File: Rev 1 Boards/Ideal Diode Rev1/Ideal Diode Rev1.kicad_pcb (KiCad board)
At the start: 2 copper layers, 78.6 x 49.5 mm, 22 parts, among them Q1 NVMFS5C404NL, U1 SN74LVC2G08, U2 LM74700

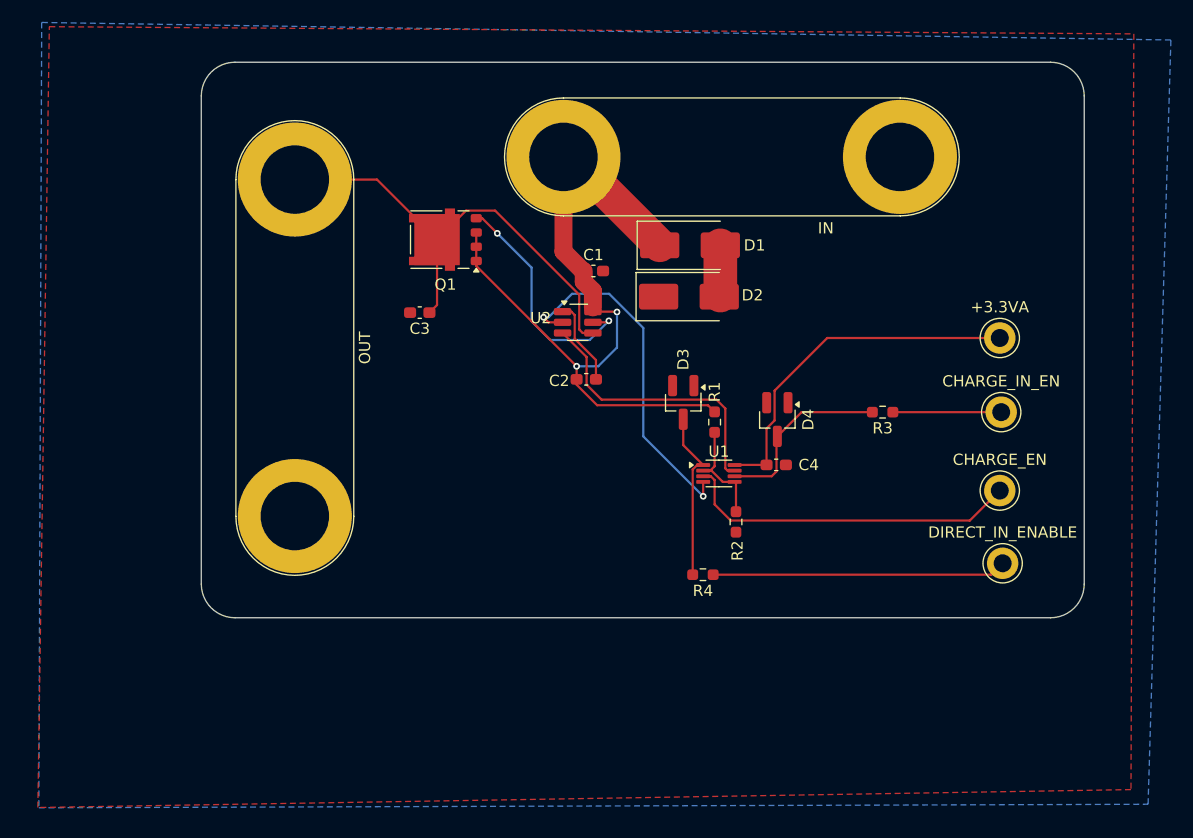
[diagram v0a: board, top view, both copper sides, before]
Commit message: ideal diode review 3 changes
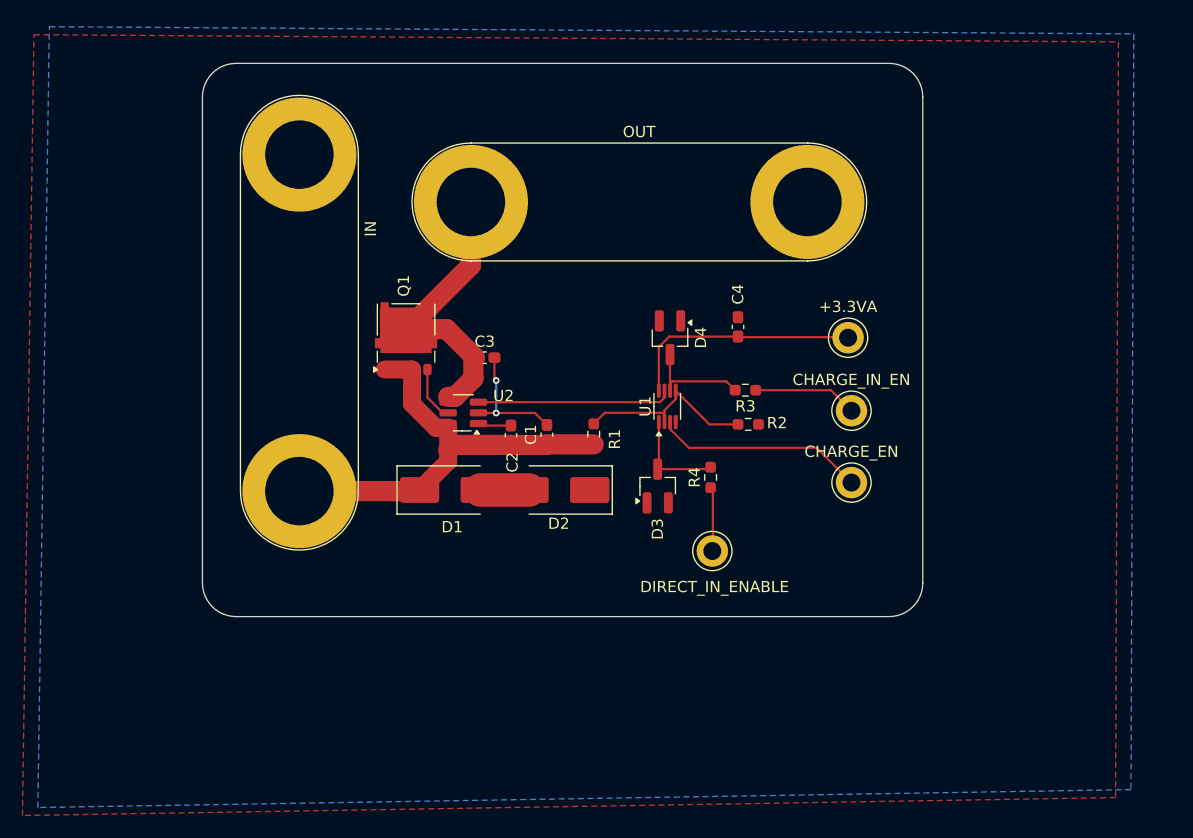
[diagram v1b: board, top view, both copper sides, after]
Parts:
- moved IN 37.9 mm to (59.8, 57.5), turned to 90 degrees
- moved D1 30.5 mm to (73.2, 57.4)
- moved DIRECT_IN_ENABLE 25.9 mm to (96.6, 62.8)
- moved G*** 23.8 mm to (90.9, 32.4)
- moved D2 20.7 mm to (82.9, 57.4), turned to 180 degrees
- moved OUT 15.8 mm to (75.1, 31.7), turned to 0 degrees
- moved C1 15.2 mm to (81.8, 52.4), turned to 90 degrees
- moved +3.3VA 13.5 mm to (108.7, 43.8)
- moved CHARGE_IN_EN 13.3 mm to (109.0, 50.3)
- moved CHARGE_EN 13.2 mm to (109.0, 56.7)
- moved U2 13.0 mm to (74.4, 50.5), turned to 180 degrees
- moved C4 12.8 mm to (98.9, 42.8), turned to 90 degrees
- moved R3 12.4 mm to (99.5, 48.5)
- moved D4 12.0 mm to (92.8, 43.8)
- moved R1 10.8 mm to (86.0, 52.4), turned to 90 degrees
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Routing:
- net /Ideal Diode/IN: track 68.0 -> 40.1 mm, vias 2 -> 0
- net /Ideal Diode/DIRECT_IEN: track 26.2 -> 5.75 mm
- net GNDPWR: track 31.4 -> 11.5 mm
- net /Ideal Diode/OUT: track 42.9 -> 25.9 mm
- net /Ideal Diode/GATE: track 21.5 -> 4.91 mm, vias 2 -> 0
- net /Ideal Diode/CHARGING_EN: track 30.4 -> 18.8 mm
- net +3.3VA: track 31.8 -> 21.2 mm
- net /Ideal Diode/DIRECT_EN: track 25.0 -> 17.4 mm
- net /Ideal Diode/V_{ON}: track 10.8 -> 17.4 mm
- net /Ideal Diode/C_CLIP: track 16.4 -> 10.1 mm
- net /Ideal Diode/D_CLIP: track 15.3 -> 9.02 mm
- net /Ideal Diode/VCAP: track 7.72 -> 2.97 mm
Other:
- board size 78.6 x 49.5 mm -> 64.2 x 49.3 mm
